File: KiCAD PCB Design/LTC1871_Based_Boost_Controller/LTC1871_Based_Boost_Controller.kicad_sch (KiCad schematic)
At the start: 13 parts, among them Q2 NMOS, U1 LTC1871EMS-7-PBF

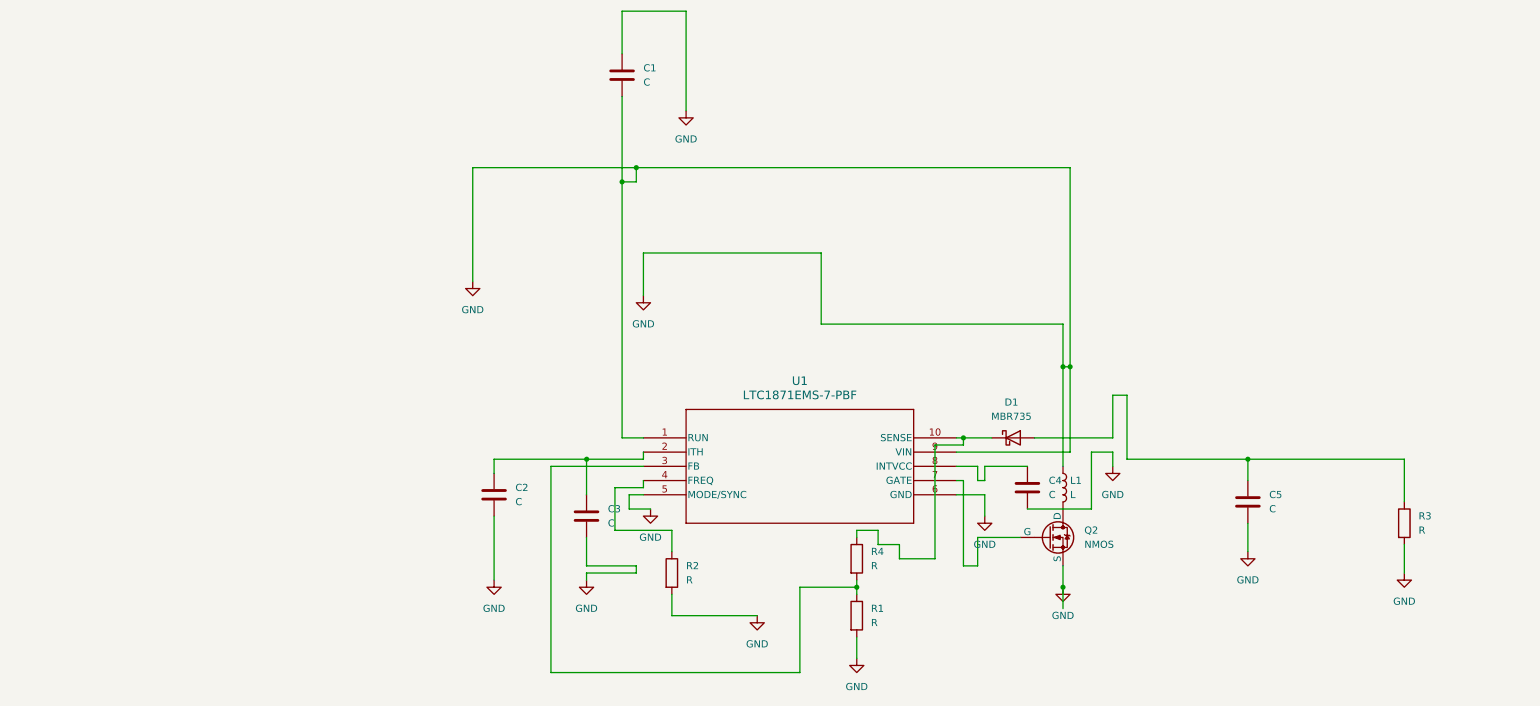
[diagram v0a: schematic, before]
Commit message: Auto-sync from Fortune at 2026-04-08 23:49:32
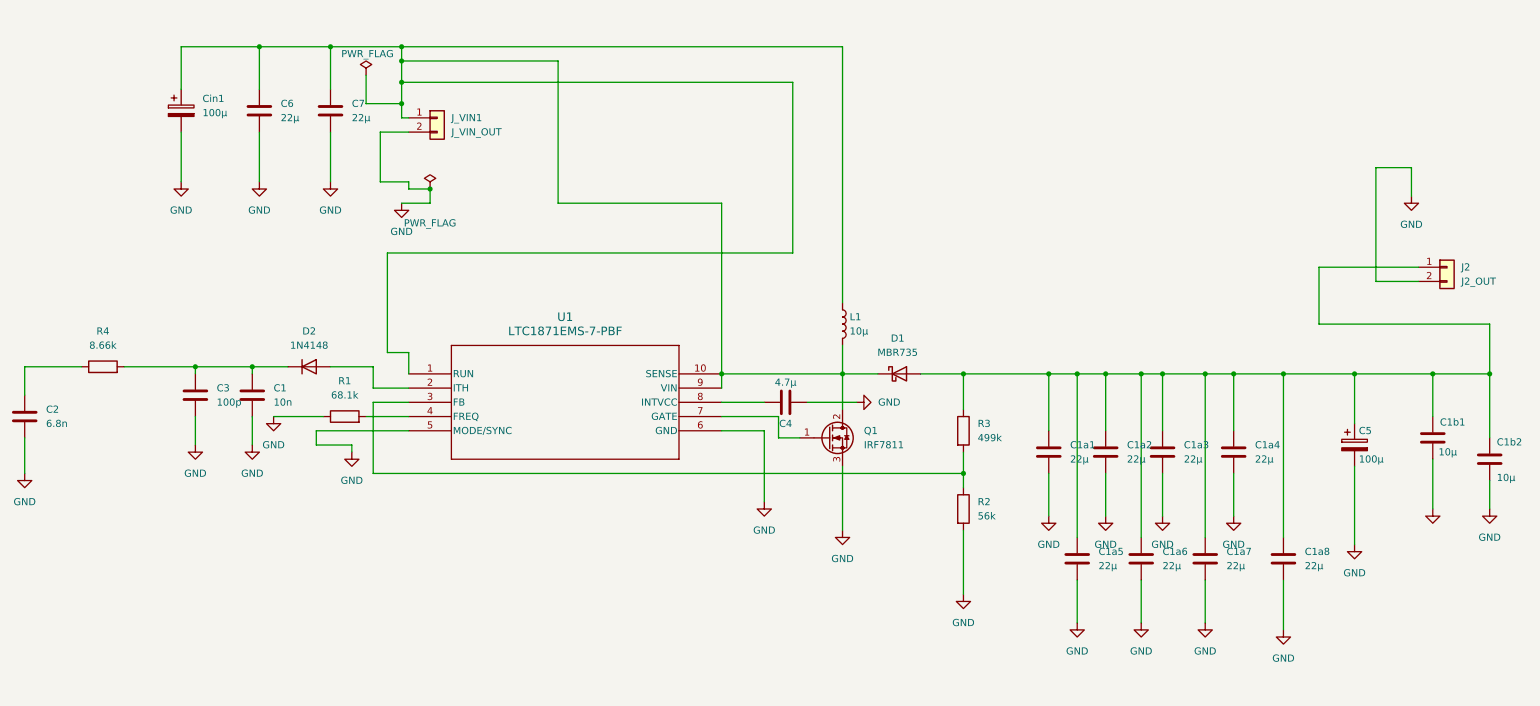
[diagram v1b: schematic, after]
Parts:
- removed C5: C, symbol Device:C
- removed D1: MBR735, Package_TO_SOT_THT:TO-220-2_Vertical, symbol Diode:MBR735
- removed Q2: NMOS, symbol Simulation_SPICE:NMOS
- added C1a1, C1a2, C1a3, C1a4, C1a5, C1a6, C1a7, C1a8, C6, C7: 22µ, Capacitor_SMD:C_1206_3216Metric, symbol Device:C
- added C1b1, C1b2: 10µ, Capacitor_SMD:C_0805_2012Metric, symbol Device:C
- added C5, Cin1: 100µ, Capacitor_THT:CP_Radial_D8.0mm_P3.50mm, symbol Device:C_Polarized
- added D1: MBR735, Diode_THT:D_DO-201AD_P15.24mm_Horizontal, symbol Device:D_Schottky
- added D2: 1N4148, Diode_SMD:D_SOD-323_HandSoldering, symbol Device:D
- added J2: J2_OUT, Connector_PinHeader_2.54mm:PinHeader_1x02_P2.54mm_Vertical, symbol Connector_Generic:Conn_01x02
- added J_VIN1: J_VIN_OUT, Connector_PinHeader_2.54mm:PinHeader_1x02_P2.54mm_Vertical, symbol Connector_Generic:Conn_01x02
- added Q1: IRF7811, Package_SO:SOIC-8_3.9x4.9mm_P1.27mm, symbol Transistor_FET:Q_NMOS_GDS
- C1: value C -> 10n; footprint (none) -> Capacitor_SMD:C_0805_2012Metric
- C2: value C -> 6.8n; footprint (none) -> Capacitor_SMD:C_0805_2012Metric
- C3: value C -> 100p; footprint (none) -> Capacitor_SMD:C_0805_2012Metric
- C4: value C -> 4.7µ; footprint (none) -> Capacitor_SMD:C_0805_2012Metric
- L1: value L -> 10µ; footprint (none) -> Inductor_SMD:L_Coilcraft_XAL6060-XXX
- R1: value R -> 68.1k; footprint (none) -> Resistor_SMD:R_0805_2012Metric
- R2: value R -> 56k; footprint (none) -> Resistor_SMD:R_0805_2012Metric
- R3: value R -> 499k; footprint (none) -> Resistor_SMD:R_0805_2012Metric
- R4: value R -> 8.66k; footprint (none) -> Resistor_SMD:R_0805_2012Metric
- U1: footprint MSOP-10_MS_LIT -> Package_SO:MSOP-10_3x3mm_P0.5mm
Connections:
- net GND: now also R1.1, C1a1.2, C1a2.2, C1a3.2, C1a4.2, C1a5.2, C1a6.2, C1a7.2, C1a8.2, C1b1.2, C1b2.2, C5.2, C6.2, C7.2, Cin1.2, J2.2 (Pin_2), J_VIN1.2 (Pin_2), Q1.3 (S); no longer C1.1, L1.1, R1.2, R3.2, U1.1 (RUN), U1.9 (VIN)
- net at R3.1: now also C1a1.1, C1a2.1, C1a3.1, C1a4.1, C1a5.1, C1a6.1, C1a7.1, C1a8.1, C1b1.1, C1b2.1, C5.1, D1.2 (A), J2.1 (Pin_1)
- net at L1.2: now also L1.1, U1.1 (RUN), U1.10 (SENSE), U1.9 (VIN), C6.1, C7.1, Cin1.1, D1.1 (K), J_VIN1.1 (Pin_1), Q1.2 (D)
- net at R4.1: now also C2.1; no longer U1.10 (SENSE)
- net at R2.1: now also R3.2, U1.3 (FB); no longer U1.4 (FREQ)
- net at U1.7 (GATE): now also Q1.1 (G)
- new net: C1.1, C3.1, D2.1 (K), R4.2
- new net: D2.2 (A), U1.2 (ITH)
- new net: R1.2, U1.4 (FREQ)
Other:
- moved on the sheet: U1
